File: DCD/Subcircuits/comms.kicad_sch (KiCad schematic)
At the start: 14 parts, among them J1 UMPS-04-03.5-G-VT-SM-WT, J2 UMPS-04-03.5-G-VT-SM-WT, J3 UMPS-04-03.5-G-VT-SM-WT, J4 UMPS-04-03.5-G-VT-SM-WT, J5 Conn_02x04_Top_Bottom

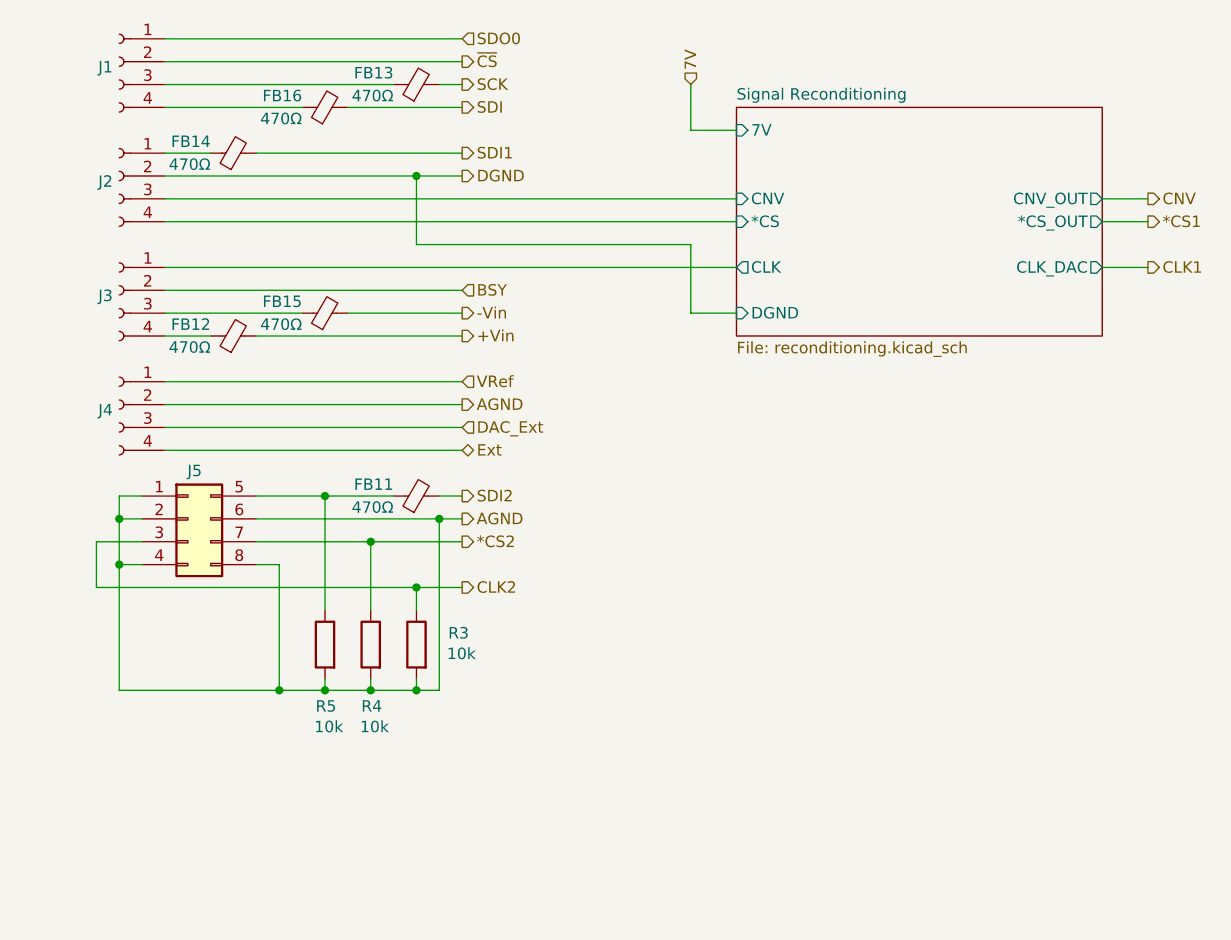
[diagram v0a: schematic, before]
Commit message: Bodges
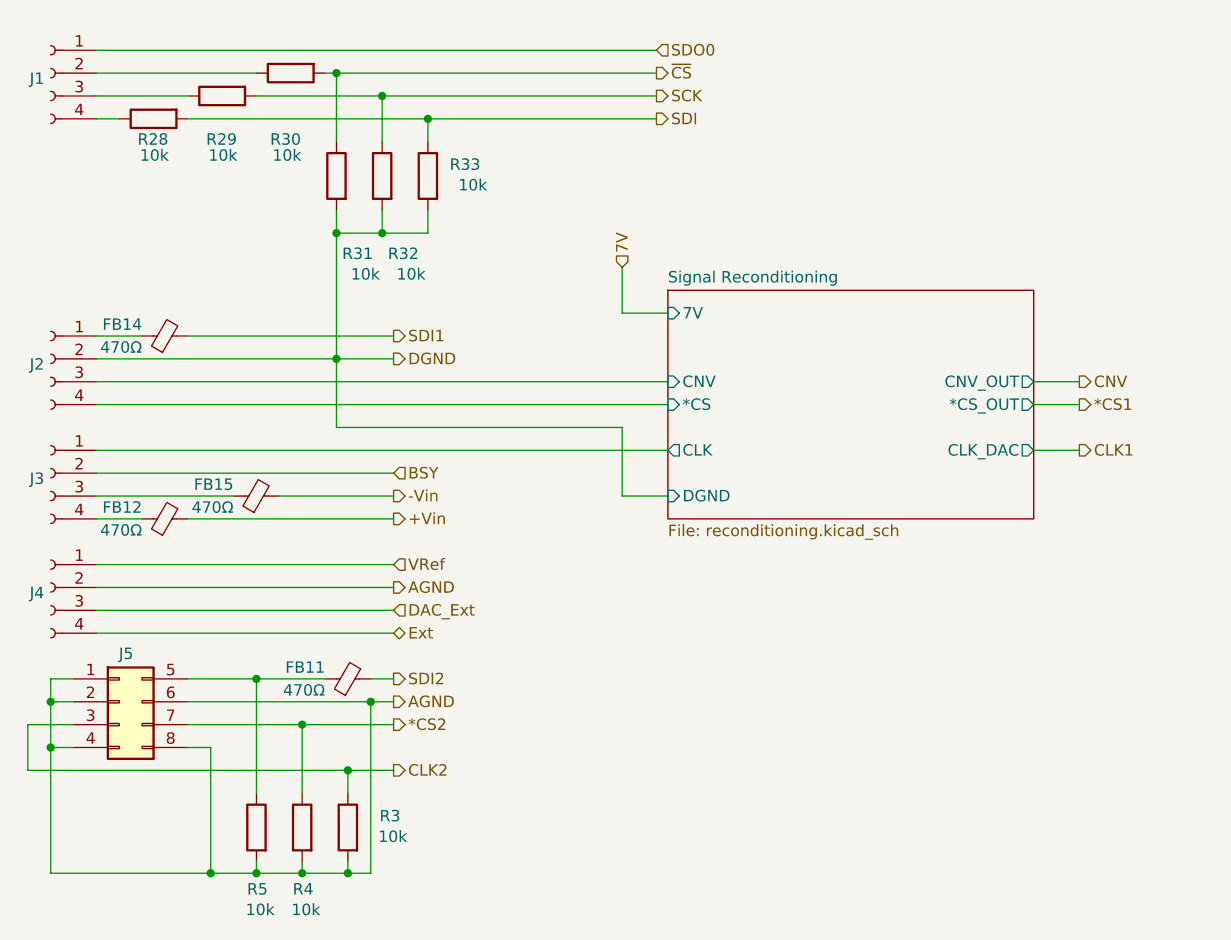
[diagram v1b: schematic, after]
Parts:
- removed FB13, FB16: 470Ω, Inductor_SMD:L_0603_1608Metric, symbol Device:FerriteBead_Small
- added R28, R29, R30, R31, R32, R33: 10k, Resistor_SMD:R_0603_1608Metric, symbol Device:R
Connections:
- net DGND: now also R31.2, R32.2, R33.2
- net SCK: now also R29.2, R32.1
- net SDI: now also R28.2, R33.1
- net ~{CS}: now also R30.2, R31.1; no longer J1.2 (Pin_2)
- net at J1.3 (Pin_3): now also R29.1
- net at J1.4 (Pin_4): now also R28.1
- new net: J1.2 (Pin_2), R30.1
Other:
- moved on the sheet: FB11, FB12, FB14, FB15, J1, J2, J3, J4, J5, R3, R4, R5
